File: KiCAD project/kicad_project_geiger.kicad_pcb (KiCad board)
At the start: 2 copper layers, 66.8 x 104.8 mm, 66 parts, among them P4 I ROVER, P7 BATTERY, Q1 2SC1815, Q2 2SC1815, SW1 SWITCH_INV, SW2 SW_DIP_3, SW4 2MD3T2B2M2RE, U1 FGPMMOPA6H, U10 MIC5205, U11 piezo_buzzer, U12 stereo_audio_socket, U2 MAX1555, U3 XBee, U4 OLED-PCB, U5 SD_CARD_SLOT, U6 MCP1826S, U7 RedBear, U8 LSM303C, U9 LM3880

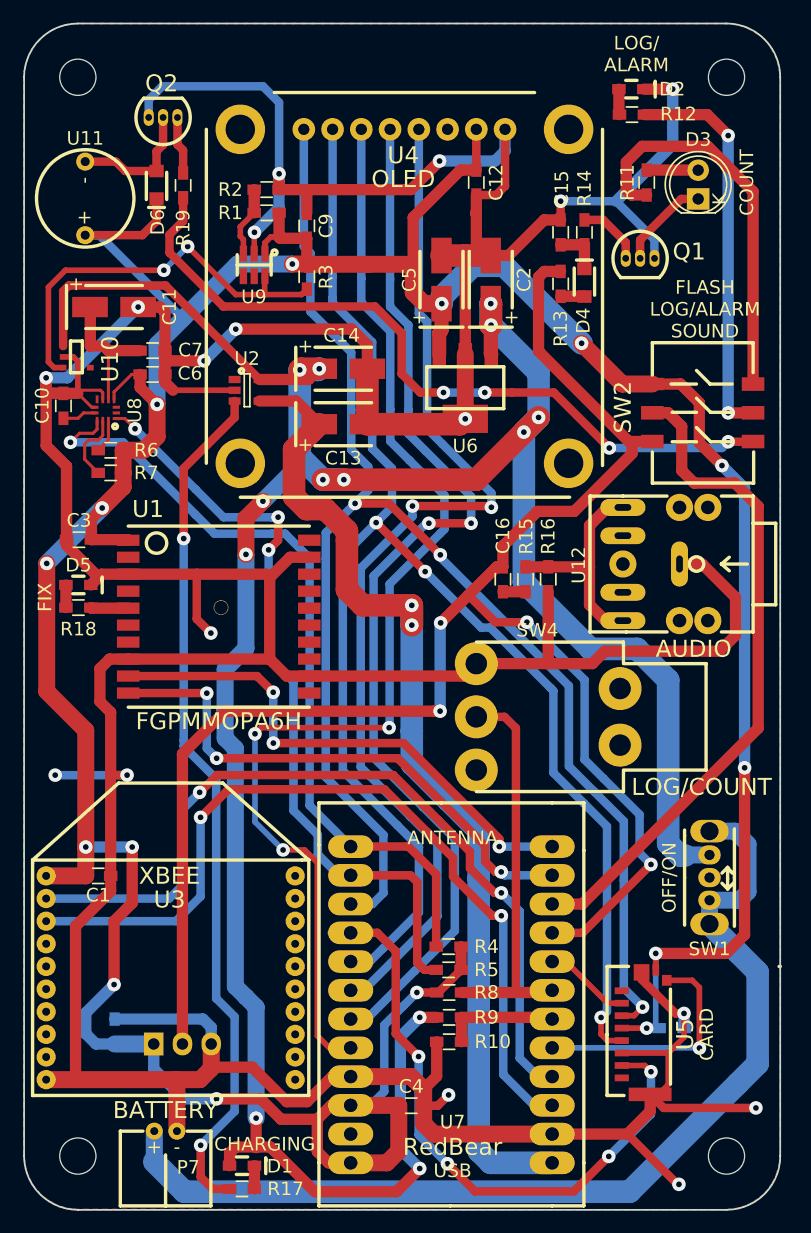
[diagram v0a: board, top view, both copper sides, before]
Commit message: Update
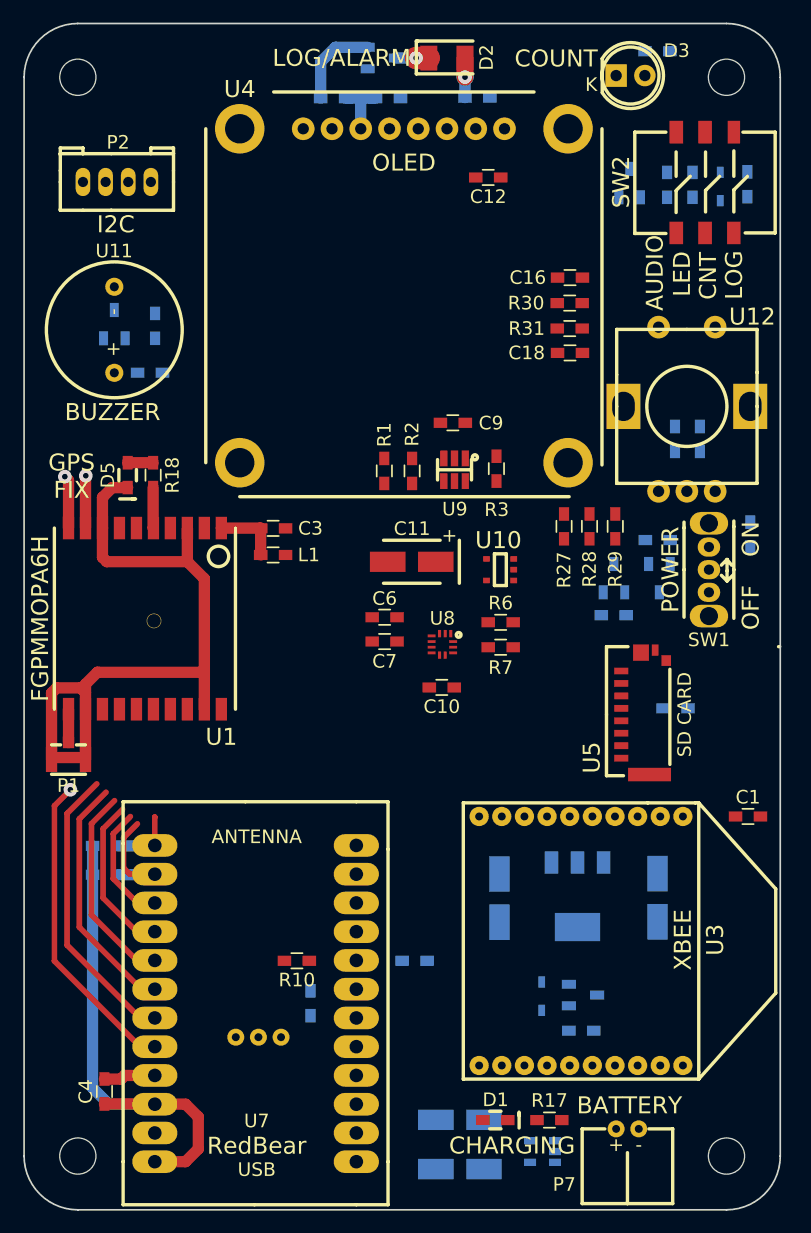
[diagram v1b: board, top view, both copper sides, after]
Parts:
- removed G***: LOGO, OPENHARDWARE:OSHWLOGO1.5IN
- removed SW4: 2MD3T2B2M2RE, TSM102C3_toggle_switch_tme:TSM102C3_toggle_switch
- added C18: 10nF, RedBear:R_0603_HandSoldering, F.Cu at (160.7, 80.2)
- added L1: Ferrite, RedBear:R_0603_HandSoldering, F.Cu at (134.5, 98.1)
- added P1: uFL_conn, UFL-R-SMT:U.FL-R-SMT, F.Cu at (116.4, 116.1)
- added P2: I2C_connector, DIP Grove 4P-2.0:DIP_Grove_4P-2_0, F.Cu at (117.7, 65.1)
- added Q3: RSR010N10FHATL, sot_32_standard:SOT-23, B.Cu at (164.6, 100.1)
- added Q4: ZXMP6A13F, sot_32_standard:SOT-23, B.Cu at (168.6, 100.1)
- added Q5: BC847C, sot_32_standard:SOT-23, B.Cu at (166.0, 65.2)
- added Q6: RSR010N10FHATL, sot_32_standard:SOT-23, B.Cu at (144.1, 54.2)
- added R20: 68R, RedBear:R_0603_HandSoldering, B.Cu at (152.5, 57.7)
- added R24: 0K, RedBear:R_0603_HandSoldering, B.Cu at (144.6, 57.7)
- added R25: 0K, RedBear:R_0603_HandSoldering, B.Cu at (139.8, 57.7)
- added R26: 0R, RedBear:R_0603_HandSoldering, B.Cu at (123.6, 82.0)
- added R27: 10K, RedBear:R_0603_HandSoldering, F.Cu at (160.2, 95.5)
- added R28: 10K, RedBear:R_0603_HandSoldering, F.Cu at (162.4, 95.5)
- added R29: 10K, RedBear:R_0603_HandSoldering, F.Cu at (164.7, 95.5)
- added R30: 10K, RedBear:R_0603_HandSoldering, F.Cu at (160.7, 75.8)
- added R31: 10K, RedBear:R_0603_HandSoldering, F.Cu at (160.7, 78.1)
- added R32: 10K, RedBear:R_0603_HandSoldering, B.Cu at (170.0, 87.8)
- added R33: 10K, RedBear:R_0603_HandSoldering, B.Cu at (172.2, 87.8)
- C13, C14, C15, C2, C5, R11, R13, R4, R5, R9, U2, U6: moved to B.Cu
- C16: value 100nF -> 10nF
- D2: footprint RedBear:LED_0603_HandSoldering -> KPD-3224SURCK:KPD-3224SURCK
- D3: value BLUE -> GREEN; footprint LEDs:LED-5MM -> MCL053SGC:MCL053SGC
- D4: footprint RedBear:1N4148 -> SOD-323_standard:SOD-323; moved to B.Cu
- D6: value 1N4148 -> BAT20J; footprint RedBear:1N4148 -> SOD-323_standard:SOD-323; moved to B.Cu
- P4: footprint Socket_Strips:Socket_Strip_Angled_1x03 -> B3B-PH-SM4-TB_IROVER_CONNECTOR:B3B-PH-SM4-TB_IROVER_CONNECTOR
- Q1: value 2SC1815 -> ZXMP6A13F; footprint 2SC1815:TO-92_Inline_Narrow_Oval -> sot_32_standard:SOT-23; moved to B.Cu
- Q2: value 2SC1815 -> RSR010N10FHATL; footprint 2SC1815:TO-92_Inline_Narrow_Oval -> sot_32_standard:SOT-23; moved to B.Cu
- R12: value 1K -> 10K; moved to B.Cu
- R14: value 100K -> 51K; moved to B.Cu
- R15: value 47K -> 10K; moved to B.Cu
- R16: value 4.7K -> 10K; moved to B.Cu
- R19: value 180K -> 10K; moved to B.Cu
- R8: value 10K -> 100K; moved to B.Cu
- U11: value piezo_buzzer -> buzzer; footprint CEM-1203(42)_piezo_buzzer:CEM-1203(42) -> LD-BZEG-1205:LD-BZEG-1205
- U12: value stereo_audio_socket -> rotary_encoder; footprint CLIFF_ELECTRONIC_COMPONENTS_FC68131_PhoneAudioConnector:CLIFF_ELECTRONIC_COMPONENTS_FC68131_PhoneAudioConnector -> rotary_enc_bourns_EC12R-4215F-S0024:rotary_enc_bourns_EC12R-4215F-S0024
- U7: footprint RedBear -> RedBear:RedBear
- moved D6 79.3 mm to (158.2, 137.0), turned to 270 degrees
- moved U2 72.1 mm to (158.3, 150.8), turned to 180 degrees
- moved C14 67.1 mm to (151.0, 148.0), turned to 180 degrees
- moved C13 66.6 mm to (151.0, 152.3), turned to 180 degrees
- moved Q1 65.2 mm to (161.9, 136.9), turned to 90 degrees
- moved R19 58.8 mm to (176.6, 96.3)
- moved C5 57.8 mm to (168.4, 128.3), turned to 270 degrees
- moved C1 57.6 mm to (176.4, 121.2)
- moved U3 56.5 mm to (170.7, 121.2), turned to 270 degrees
- moved C2 54.6 mm to (154.5, 128.4), turned to 270 degrees
- moved R12 46.1 mm to (124.1, 77.8), turned to 270 degrees
- moved U6 46.0 mm to (161.4, 125.4), turned to 0 degrees
- moved U10 44.9 mm to (155.7, 100.3), turned to 90 degrees
- moved C10 41.7 mm to (149.4, 109.8), turned to 180 degrees
- moved P7 40.8 mm to (165.8, 148.8)
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- renumbered REF** to ?
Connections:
- C16 pad 1: Net-(C16-Pad1) -> GND
- C16 pad 2: IROVER -> ENC_B
- C2 pad 1: VBAT -> LDO
- C3 pad 2: +3V3 -> Net-(C3-Pad2)
- D2 pad 1: GND -> Net-(D2-Pad1)
- D6 pad 1: +3V3 -> PWR
- D6 pad 2: Net-(D6-Pad2) -> VUSB
- P7 pad 1: Net-(P7-Pad1) -> VBAT
- Q1 pad 1: GND -> VUSB
- Q1 pad 2: Net-(D3-Pad1) -> PWR
- Q1 pad 3: Net-(Q1-Pad3) -> VBAT
- Q2 pad 1: GND -> IROVER
- Q2 pad 2: Net-(D6-Pad2) -> GND
- R10 pad 1: Net-(R10-Pad1) -> BAT_MEASURE
- R11 pad 1: Net-(D3-Pad2) -> CNT_LED
- R11 pad 2: Net-(R11-Pad2) -> Net-(D3-Pad2)
- R12 pad 1: Net-(D2-Pad2) -> GND
- R12 pad 2: Net-(R12-Pad2) -> IROVER
- R14 pad 1: Net-(Q1-Pad3) -> Net-(Q5-Pad1)
- R15 pad 1: Net-(C16-Pad1) -> GND
- R15 pad 2: Net-(R15-Pad2) -> PWR_ON
- R16 pad 1: Net-(R15-Pad2) -> Net-(Q3-Pad3)
- R16 pad 2: GND -> PWR
- R18 pad 1: Net-(D5-Pad2) -> Net-(R18-Pad1)
- R18 pad 2: Net-(R18-Pad2) -> Net-(D5-Pad2)
- R19 pad 1: Net-(R19-Pad1) -> GND
- R19 pad 2: Net-(Q2-Pad3) -> PWR_OFF
- R8 pad 1: +3V3 -> VUSB
- R8 pad 2: LOG_CNT_SEL -> GND
- R9 pad 2: Net-(R10-Pad1) -> BAT_MEASURE
- SW1 pad 1: (no net) -> LDO
- SW1 pad 2: VBAT -> PWR
- SW1 pad 3: Net-(P7-Pad1) -> PWR_OFF
- SW2 pad 2: LOG_ALARM -> +3V3
- SW2 pad 3: IROVER -> +3V3
- SW2 pad 4: Net-(R19-Pad1) -> PIEZO
- SW2 pad 5: Net-(R12-Pad2) -> CNT_LED
- SW2 pad 6: Net-(R11-Pad2) -> LOG_LED
- U1 pad 1: +3V3 -> Net-(C3-Pad2)
- U1 pad 11: (no net) -> Net-(P1-Pad1)
- U1 pad 4: (no net) -> VBAT
- U1 pad 5: Net-(R18-Pad2) -> Net-(R18-Pad1)
- U11 pad 1: +3V3 -> Net-(R26-Pad2)
- U11 pad 2: Net-(D6-Pad2) -> Net-(Q2-Pad3)
- U12 pad 2: Net-(R15-Pad2) -> ENC_SW
- U12 pad 3: Net-(R15-Pad2) -> Net-(R31-Pad2)
- U4 pad 1: SPI_MOSI -> I2C_SDA
- U4 pad 2: SPI_SCK -> I2C_SCL
- U4 pad 3: LCD_DC -> Net-(R24-Pad2)
- U4 pad 5: LCD_CS -> GND
- U6 pad 1: VBAT -> LDO
- U7 pad 15: LOG_ALARM -> IROVER
- U7 pad 16: IROVER -> ENC_SW
- U7 pad 17: CS_LOG -> BAT_MEASURE
- U7 pad 18: LOG_CNT_SEL -> PWR_OFF
- U7 pad 19: Net-(R10-Pad1) -> ENC_A
- U7 pad 20: CD_LOG -> ENC_B
- U7 pad 6: LCD_CS -> CS_LOG
- U7 pad 7: LCD_RST -> PWR_ON
- U7 pad 8: LCD_DC -> LCD_RST
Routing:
- net GND: track 494.6 -> 74.1 mm, vias 17 -> 0
- net +3V3: track 338.9 -> 43.4 mm, vias 15 -> 0
- net VBAT: track 239.0 -> 0.00 mm, vias 13 -> 0
- net IROVER: track 148.4 -> 0.00 mm, vias 4 -> 0
- net SPI_MOSI: track 135.8 -> 10.7 mm, vias 3 -> 0
- net SPI_SCK: track 141.3 -> 18.2 mm, vias 3 -> 0
- net LCD_DC: track 103.5 -> 0.00 mm, vias 3 -> 0
- net LCD_CS: track 96.1 -> 0.00 mm, vias 2 -> 0
- net VUSB: track 90.2 -> 0.00 mm, vias 2 -> 0
- net Net-(P7-Pad1): track 89.8 -> 0.00 mm
- net Net-(R17-Pad2): track 76.5 -> 0.00 mm, vias 2 -> 0
- net TX_XBEE: track 74.3 -> 0.00 mm, vias 2 -> 0
- net RX_XBEE: track 72.6 -> 0.00 mm, vias 2 -> 0
- net LCD_RST: track 95.1 -> 27.7 mm, vias 2 -> 1
- net Net-(R19-Pad1): track 66.4 -> 0.00 mm, vias 4 -> 0
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- removed copper zone on B.Cu, net GND
- removed copper zone on F.Cu, net GND
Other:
- net class Default: clearance 0.202 -> 0.21; trace_width 0.5 -> 0.4
- rule trace_clearance: 0.202 -> 0.21
- rule trace_min: 0.1905 -> 0.4
- board text added: "BUZZER"
- board text added: "CNT"
- board text added: "GPS FIX"
- board text added: "I2C"
- board text added: "LED"
- board text added: "LOG"
- board text added: "LOG/ALARM"
- board text added: "OFF"
- board text added: "ON"
- board text added: "POWER"
- board text added: "iRover"
- board text removed: "FIX"
- board text removed: "FLASH LOG/ALARM SOUND"
- board text removed: "Institute IRNAS Rače www.irnas.eu"
- board text removed: "Integrated Safecast bGeigie Nano"
- board text removed: "LOG/ ALARM"
- board text removed: "LOG/COUNT"
- board text removed: "OFF/ON"
